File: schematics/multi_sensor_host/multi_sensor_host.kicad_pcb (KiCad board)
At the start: 2 copper layers, 169 parts, among them J1 left hand 0, J10 swd, J11 stm_boot, J13 right hand 0, J14 right hand 1, J15 right hand 2, J16 right hand 3, J17 rst_mcu, J18 left hand 3, J19 left leg 0, J2 left hand 1, J20 left leg 1, J21 right lef 0, J22 right leg 1, J3 bm_cfg, J4 left hand 2, J5 tx, J6 MY_USB_B, J7 rst_bm71, J8 rx, J9 uart1, U1 TCA9548A_TSSOP, U11 MCP111, U12 BM71BLES1FC2-0B02AA, U2 TCA9548A_TSSOP, U3 TCA9548A_TSSOP, U4 MCP111, U5 TPS79333-EP, U8 MCP73812, U9 MCP1603, Y1 Crystal

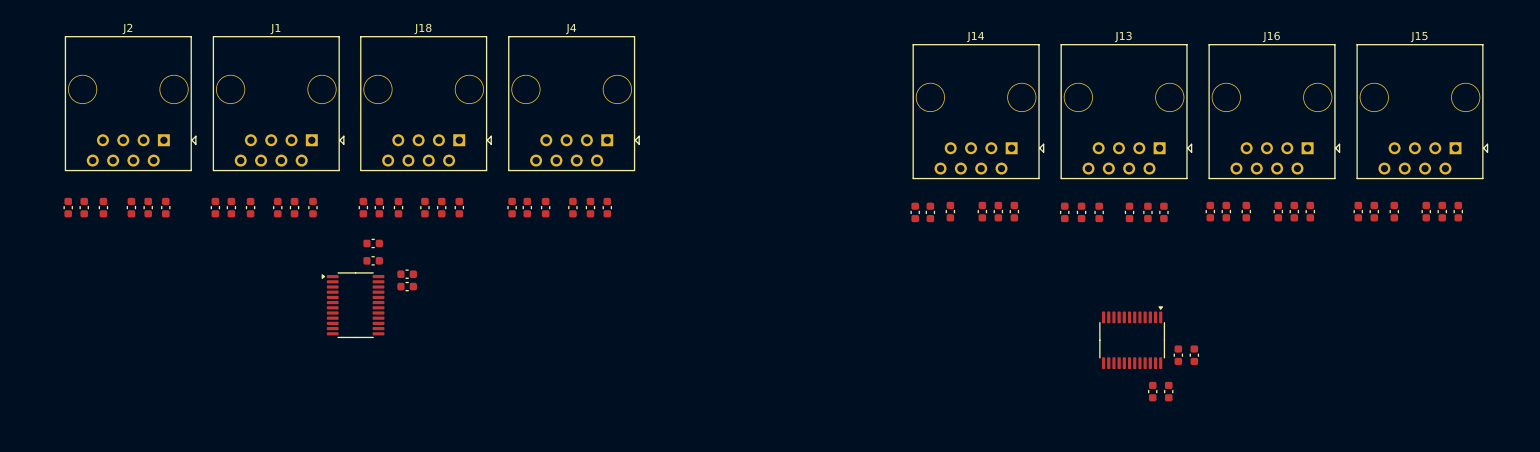
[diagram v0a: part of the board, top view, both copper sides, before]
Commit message: a
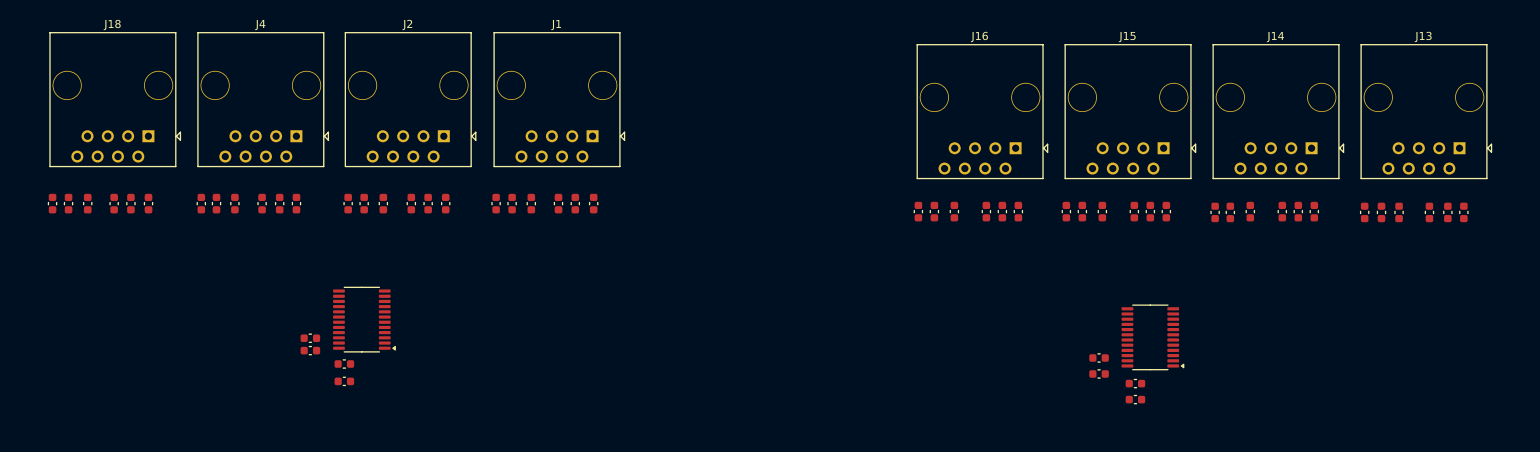
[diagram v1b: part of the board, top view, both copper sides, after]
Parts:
- moved C40 38.9 mm to (-0.76, -54.7)
- moved C41 38.9 mm to (1.24, -54.7)
- moved C44 38.9 mm to (17.8, -54.7)
- moved C45 38.9 mm to (19.7, -54.7)
- moved J18 38.9 mm to (11.2, -63.1)
- moved J4 38.9 mm to (29.7, -63.1)
- moved R14 38.9 mm to (27.6, -54.7)
- moved R15 38.9 mm to (22.0, -54.7)
- moved R16 38.9 mm to (9.04, -54.7)
- moved R17 38.9 mm to (3.64, -54.7)
- moved R22 38.9 mm to (29.7, -54.7)
- moved R23 38.9 mm to (25.4, -54.7)
- moved R24 38.9 mm to (11.2, -54.7)
- moved R25 38.9 mm to (6.94, -54.7)
- moved C56 37.5 mm to (163.3, -53.6)
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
